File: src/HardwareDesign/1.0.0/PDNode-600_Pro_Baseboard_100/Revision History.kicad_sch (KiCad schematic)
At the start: 0 parts

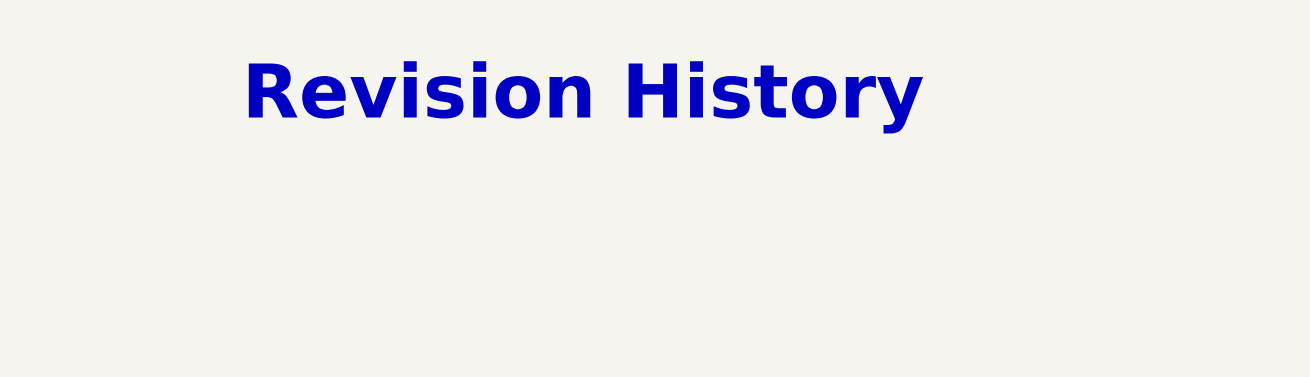
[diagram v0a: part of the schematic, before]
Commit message: baseboard development
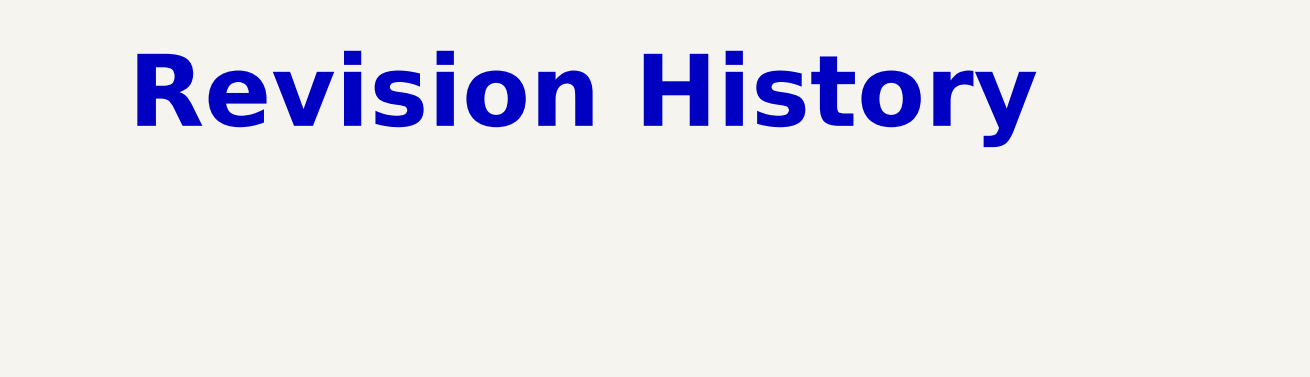
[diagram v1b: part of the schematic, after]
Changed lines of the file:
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@@
 			(font
 				(face "Times New Roman")
-				(size 6 6)
+				(size 8 8)
 				(thickness 1.2)
 				(bold yes)
-				(color 162 22 34 1)
+				(color 43 49 168 1)
 			)
 		)
